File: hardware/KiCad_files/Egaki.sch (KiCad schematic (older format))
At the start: 74 parts, among them IC1 ULN2803, U1 CONN_01X04, U2 ESP01, U3 CONN_01X04, U4 CONN_01X04, U5 CONN_01X04, U6 LM1117-SOT, X1 Screw_Terminal_1x02

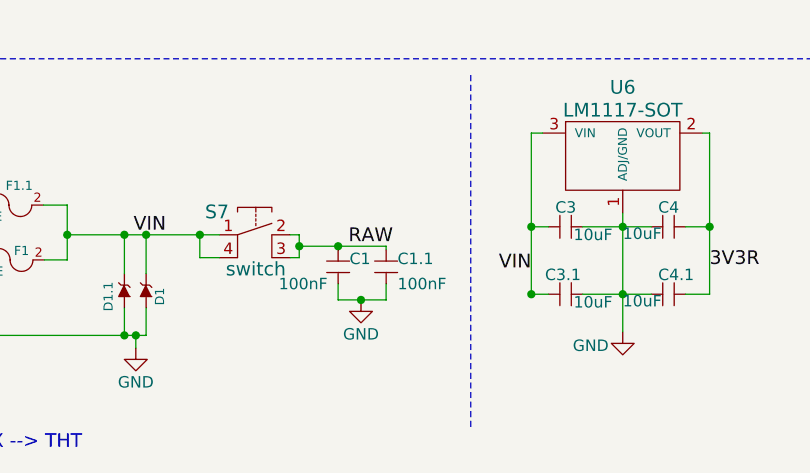
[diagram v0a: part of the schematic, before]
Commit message: Actualización a Egaki
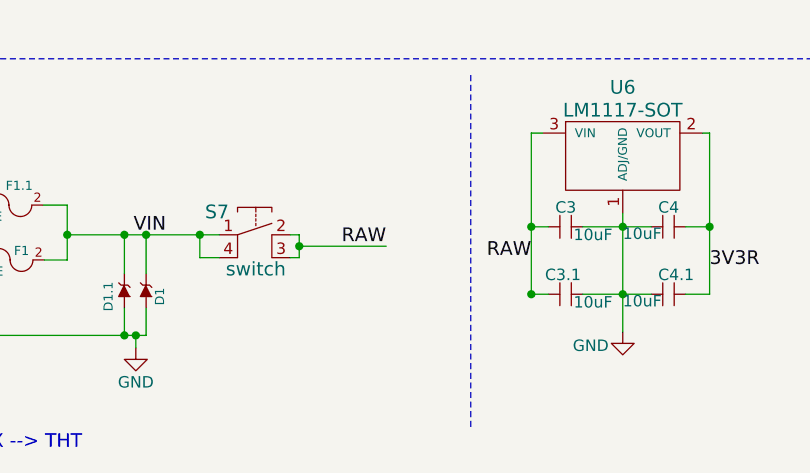
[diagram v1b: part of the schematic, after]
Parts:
- removed C1: 100nF, Capacitors_ThroughHole:C_Disc_D5.0mm_W2.5mm_P5.00mm, symbol C
- removed C1.1: 100nF, Capacitors_SMD:C_0603_HandSoldering, symbol C
- S1.1, S2.1, S3.1, S4.1, S5.1: footprint Buttons_Switches_ThroughHole:SW_PUSH_6mm -> Switch:SW_PUSH_6mm
- S7: footprint ComponentesVarios:on_off_Switch -> Switch:on_off_Switch
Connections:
- net RAW: now also C3.1.2, C3.2, U6.3 (VIN)
- net VIN: no longer C3.1.2, C3.2, U6.3 (VIN)
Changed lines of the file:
@@
 LIBS:analog
 LIBS:esp01
-LIBS:furubot_R2-cache
+LIBS:furubot_R3-cache
 EELAYER 25 0
 EELAYER END
@@
 F 0 "S5.1" H 10365 1430 60  0000 C CNN
 F 1 "switch" H 10600 1740 60  0000 C CNN
-F 2 "Buttons_Switches_ThroughHole:SW_PUSH_6mm" H 10285 1740 60  0001 C CNN
+F 2 "Switch:SW_PUSH_6mm" H 10285 1740 60  0001 C CNN
 F 3 "" H 10285 1740 60  0001 C CNN
 	1    10285 1740
@@
 F 0 "S4.1" H 10830 1435 60  0000 C CNN
 F 1 "switch" H 11065 1740 60  0000 C CNN
-F 2 "Buttons_Switches_ThroughHole:SW_PUSH_6mm" H 10750 1740 60  0001 C CNN
+F 2 "Switch:SW_PUSH_6mm" H 10750 1740 60  0001 C CNN
 F 3 "" H 10750 1740 60  0001 C CNN
 	1    10750 1740
@@
 F 0 "S2.1" H 9435 1430 60  0000 C CNN
 F 1 "switch" H 9665 1735 60  0000 C CNN
-F 2 "Buttons_Switches_ThroughHole:SW_PUSH_6mm" H 9355 1740 60  0001 C CNN
+F 2 "Switch:SW_PUSH_6mm" H 9355 1740 60  0001 C CNN
 F 3 "" H 9355 1740 60  0001 C CNN
 	1    9355 1740
@@
 F 0 "S3.1" H 9905 1430 60  0000 C CNN
 F 1 "switch" H 10135 1740 60  0000 C CNN
-F 2 "Buttons_Switches_ThroughHole:SW_PUSH_6mm" H 9820 1740 60  0001 C CNN
+F 2 "Switch:SW_PUSH_6mm" H 9820 1740 60  0001 C CNN
 F 3 "" H 9820 1740 60  0001 C CNN
 	1    9820 1740
@@
 F 0 "S1.1" H 8970 1420 60  0000 C CNN
 F 1 "switch" H 9200 1740 60  0000 C CNN
-F 2 "Buttons_Switches_ThroughHole:SW_PUSH_6mm" H 8890 1740 60  0001 C CNN
+F 2 "Switch:SW_PUSH_6mm" H 8890 1740 60  0001 C CNN
 F 3 "" H 8890 1740 60  0001 C CNN
 	1    8890 1740
@@
 $EndComp
 $Comp
-L C C1
-U 1 1 58BBB7D0
-P 3770 6855
-F 0 "C1" H 3820 6865 50  0000 L CNN
-F 1 "100nF" H 3510 6755 50  0000 L CNN
-F 2 "Capacitors_ThroughHole:C_Disc_D5.0mm_W2.5mm_P5.00mm" H 3770 6855 60  0001 C CNN
-F 3 "" H 3770 6855 60  0000 C CNN
-	1    3770 6855
-	1    0    0    -1
-$EndComp
-$Comp
-L C C1.1
-U 1 1 58BBBA67
-P 3980 6855
-F 0 "C1.1" H 4030 6865 50  0000 L CNN
-F 1 "100nF" H 4030 6755 50  0000 L CNN
-F 2 "Capacitors_SMD:C_0603_HandSoldering" H 3980 6855 60  0001 C CNN
-F 3 "" H 3980 6855 60  0000 C CNN
-	1    3980 6855
-	1    0    0    -1
-$EndComp
-$Comp
-L GND #PWR012
-U 1 1 58BBC34A
-P 3870 7025
-F 0 "#PWR012" H 3870 6775 50  0001 C CNN
-F 1 "GND" H 3870 6875 50  0000 C CNN
-F 2 "" H 3870 7025 50  0000 C CNN
-F 3 "" H 3870 7025 50  0000 C CNN
-	1    3870 7025
-	1    0    0    -1
-$EndComp
-$Comp
 L ESP01 U2
 U 1 1 58BBE9A1
@@
 Text Label 8935 3770 0    60   ~ 0
 RAW
-Text Label 3815 6790 0    60   ~ 0
+Text Label 3980 6790 2    60   ~ 0
 RAW
 Text Label 2875 6740 0    60   ~ 0
@@
 A4
 $Comp
-L GND #PWR013
+L GND #PWR012
 U 1 1 58D30B35
 P 3185 2675
-F 0 "#PWR013" H 3185 2425 50  0001 C CNN
+F 0 "#PWR012" H 3185 2425 50  0001 C CNN
 F 1 "GND" H 3185 2525 50  0000 C CNN
 F 2 "" H 3185 2675 50  0000 C CNN
@@
 F 0 "S7" H 3240 6640 60  0000 C CNN
 F 1 "switch" H 3410 6390 60  0000 C CNN
-F 2 "ComponentesVarios:on_off_Switch" H 3330 6640 60  0001 C CNN
+F 2 "Switch:on_off_Switch" H 3330 6640 60  0001 C CNN
 F 3 "" H 3330 6640 60  0001 C CNN
 	1    3330 6640
@@
 $EndComp
 $Comp
-L GND #PWR014
+L GND #PWR013
 U 1 1 58DC633A
 P 5015 7165
-F 0 "#PWR014" H 5015 6915 50  0001 C CNN
+F 0 "#PWR013" H 5015 6915 50  0001 C CNN
 F 1 "GND" H 4875 7105 50  0000 C CNN
 F 2 "" H 5015 7165 50  0000 C CNN
@@
 	1    0    0    -1
 $EndComp
-Text Label 4615 6905 2    60   ~ 0
-VIN
 Text Label 5395 6890 0    60   ~ 0
 3V3R
@@
 	2835 7060 2835 7180
 Connection ~ 2930 6740
-Wire Wire Line
-	3770 6955 3770 7025
-Wire Wire Line
-	3770 7025 3980 7025
-Wire Wire Line
-	3980 7025 3980 6955
-Connection ~ 3870 7025
 Wire Notes Line
 	4350 7580 4350 6040
@@
 	3600 6740 3560 6740
 Wire Wire Line
-	3980 6790 3980 6805
-Wire Wire Line
 	3600 6790 3980 6790
 Connection ~ 3600 6790
 Wire Wire Line
-	3770 6805 3770 6790
-Connection ~ 3770 6790
-Wire Wire Line
 	885  915  625  915
 Wire Wire Line
@@
 Text Label 1860 5695 2    60   ~ 0
 GND
+Text Label 4615 6850 2    60   ~ 0
+RAW
 $EndSCHEMATC
